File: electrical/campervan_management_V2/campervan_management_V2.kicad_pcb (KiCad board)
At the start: 4 copper layers, 169.5 x 96 mm, 172 parts, among them J1 Battery & Fuse, J10 Fans, J2 RS485, J3 Temp, J4 Output Flow Sensor, J5 Input Flow Sensor, J6 Power On/Off Switch, J7 Starter Battery, J8 Battery 2, J9 Relays, K1 G6KU-2, Q1 Q_PMOS_DGS, Q2 Q_PMOS_DGS, Q3 Q_PMOS_DGS, Q4 Q_PMOS_DGS, Q5 Q_PMOS_DGS, Q6 Q_PMOS_DGS, Q7 MMBT2222A, Q8 MMBT2222A, SW1 SW_Push, U1 MCP16311x-xMNY, U10 LM358DR2G, U11 LM358DR2G, U12 LTV-817S-TA1-C, U13 LTV-817S-TA1-C, U14 LTV-817S-TA1-C, U15 HCNR200-500E, U16 LTV-817S-TA1-C, U17 LM358DR2G, U18 LTV-817S-TA1-C, U19 LM358DR2G, U2 AMS1117-3.3, U20 LTV-817S-TA1-C, U21 LTV-817S-TA1-C, U22 HCNR200-500E, U23 LM358DR2G, U24 LTV-817S-TA1-C, U25 LTV-817S-TA1-C, U3 MCP16311x-xMNY, U4 AMS1117-3.3, U5 MAX487E, U6 LTV-817S-TA1-C, U7 LTV-817S-TA1-C, U8 LTV-817S-TA1-C, U9 HCNR200-500E

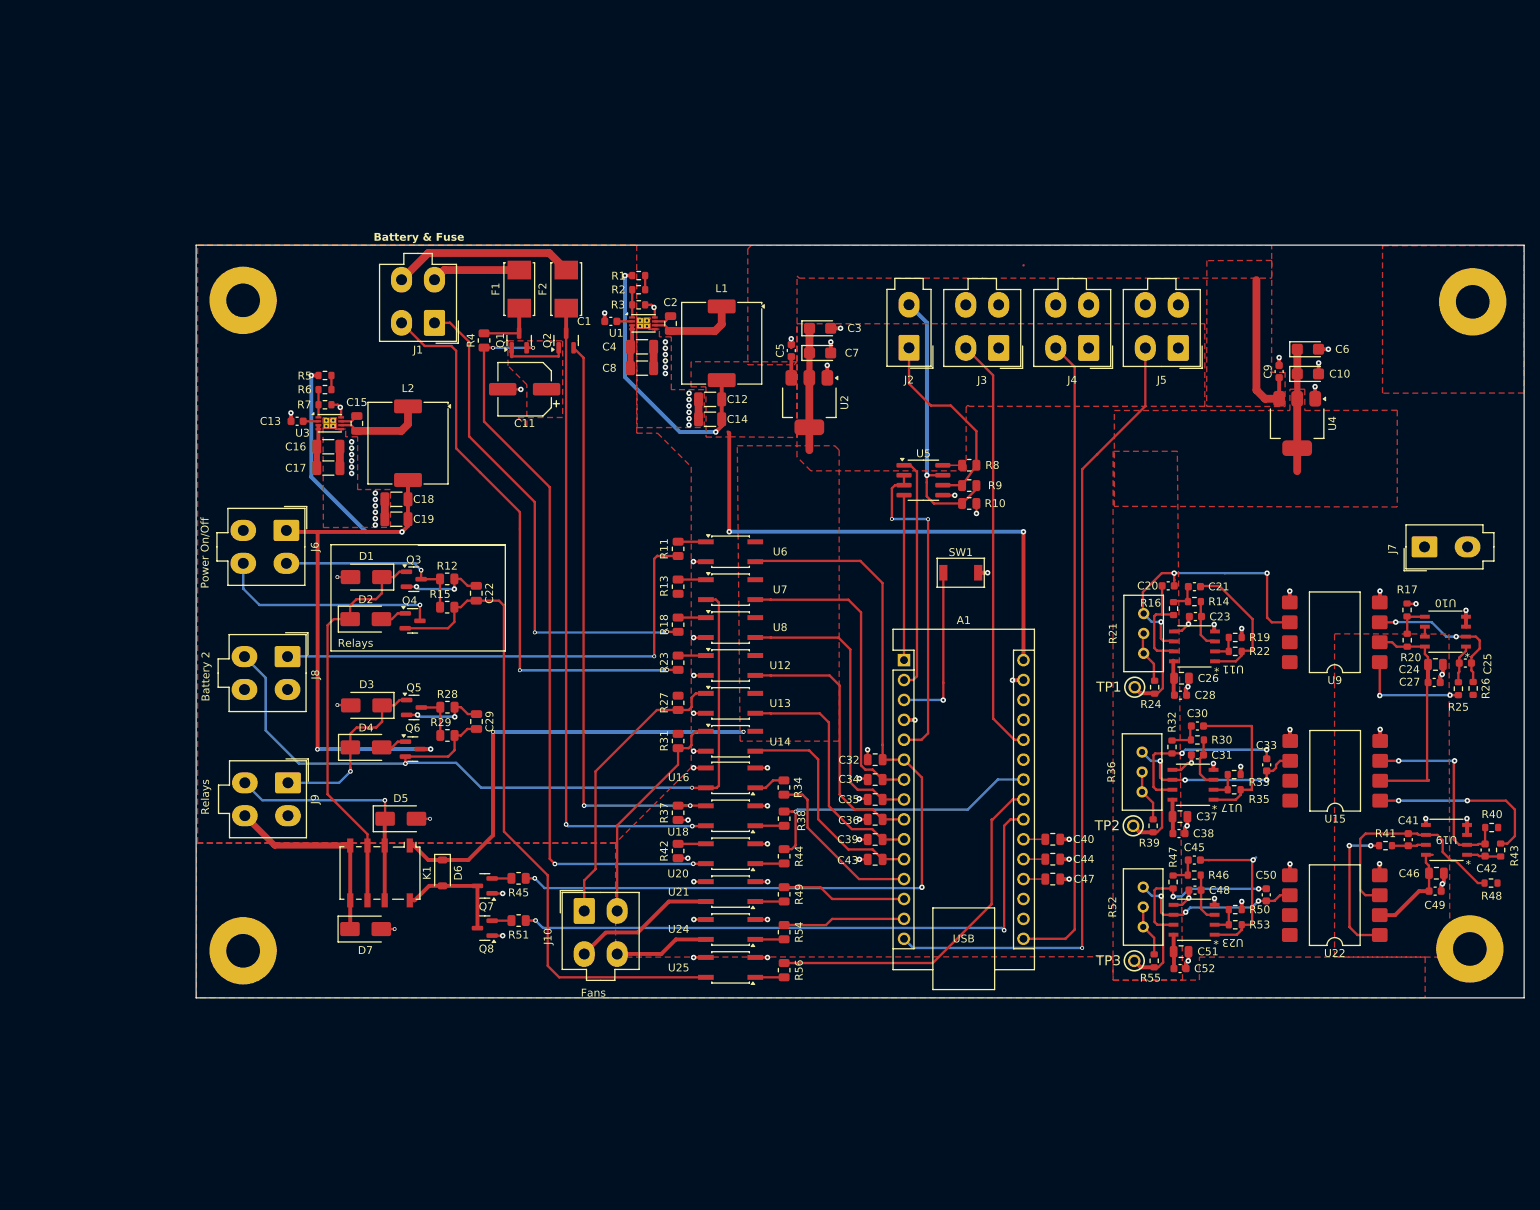
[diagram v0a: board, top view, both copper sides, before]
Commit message: Close to final design
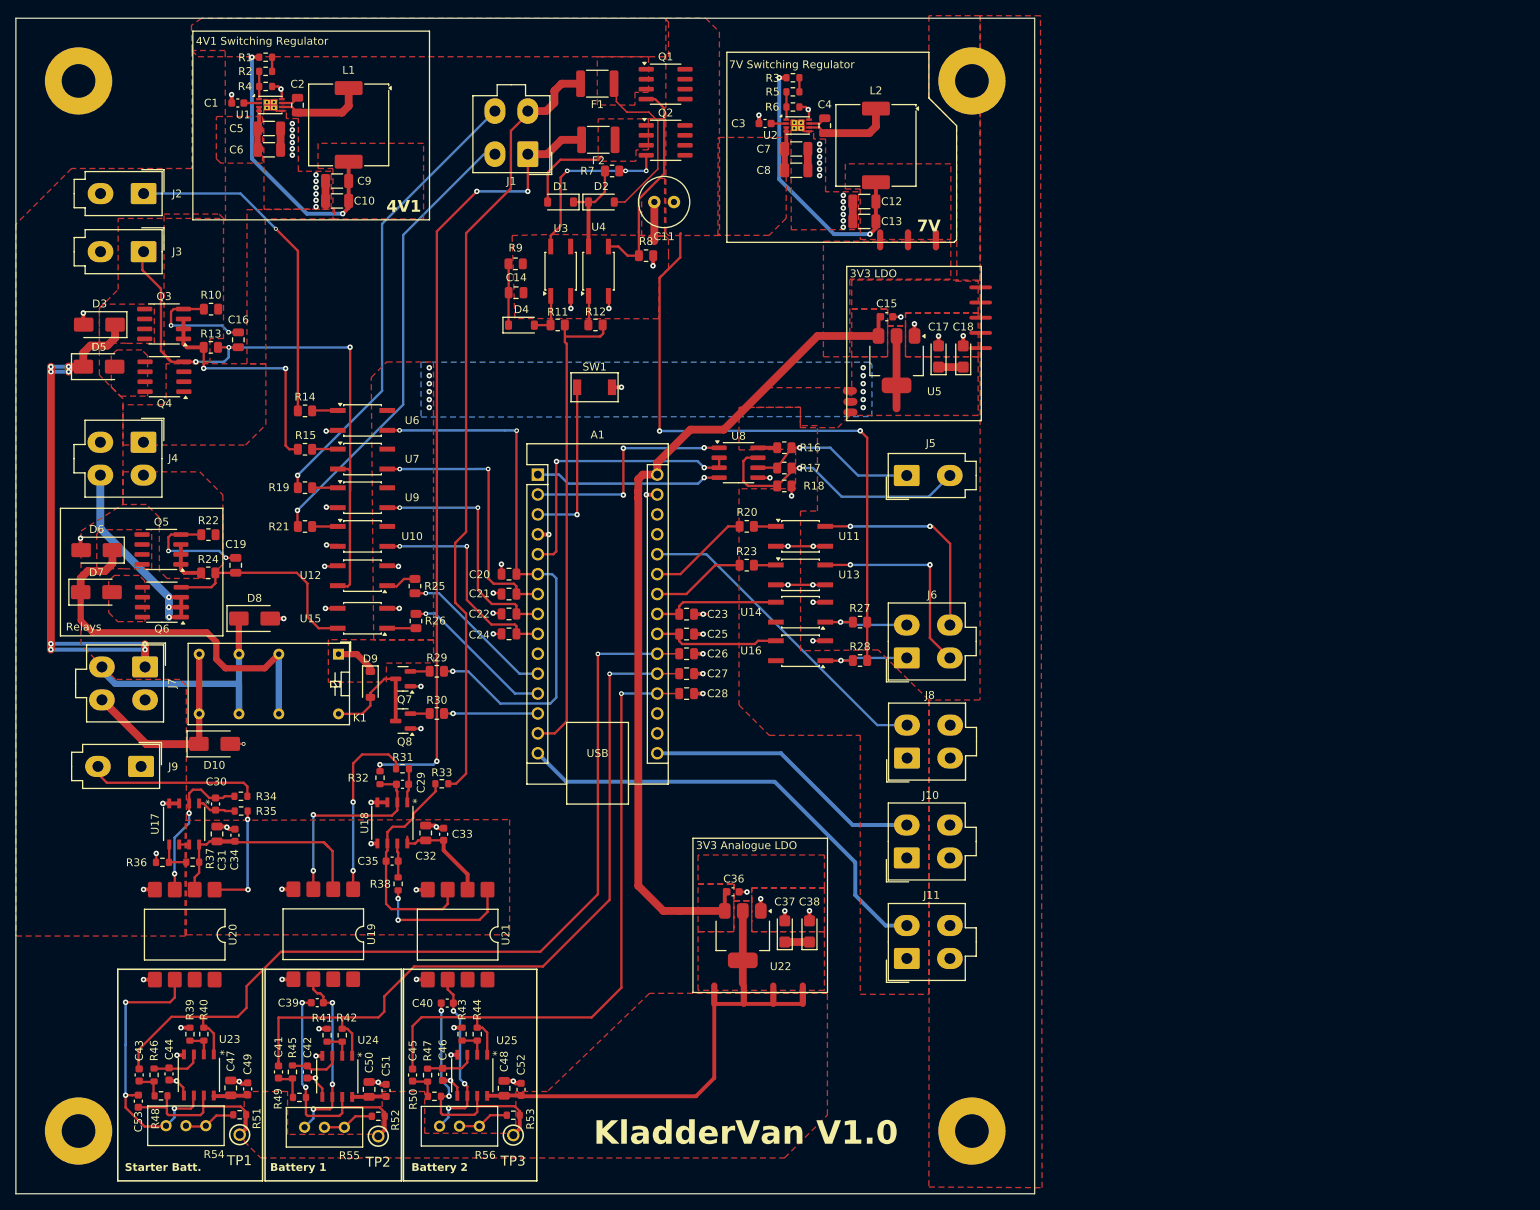
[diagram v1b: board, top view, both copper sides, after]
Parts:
- removed the J8 at (61.7, 106.5)
- removed the R42 at (111.5, 131.3)
- added C14: 220pF, Capacitor_SMD:C_0805_2012Metric, F.Cu at (90.8, 60.0)
- added D1: 1N418W, Diode_SMD:D_SOD-123, F.Cu at (96.5, 48.5)
- added D2: 1N418W, Diode_SMD:D_SOD-123, F.Cu at (101.7, 48.5)
- added D4: 1N418W, Diode_SMD:D_SOD-123, F.Cu at (91.5, 64.2)
- added J2: Battery 2, Connector_Molex:Molex_Mini-Fit_Jr_5566-02A_2x01_P4.20mm_Vertical, F.Cu at (43.3, 47.4)
- added J3: Solar Charge, Connector_Molex:Molex_Mini-Fit_Jr_5566-02A_2x01_P4.20mm_Vertical, F.Cu at (43.3, 54.8)
- added R9: 330, Resistor_SMD:R_0805_2012Metric, F.Cu at (90.8, 56.3)
- C11: footprint Capacitor_SMD:CP_Elec_6.3x5.9 -> Capacitor_THT:C_Radial_D6.3mm_H11.0mm_P2.50mm
- F1: renamed from F2; footprint Fuse:Fuseholder_Littelfuse_Nano2_157x -> Fuse:Fuse_1812_4532Metric
- F2: renamed from F1; footprint Fuse:Fuseholder_Littelfuse_Nano2_157x -> Fuse:Fuse_1812_4532Metric
- K1: value G6KU-2 -> G5V-2; footprint Relay_SMD:Relay_DPDT_Omron_G6K-2F-Y -> Relay_THT:Relay_DPDT_Omron_G5V-2
- Q1, Q2, Q3, Q4, Q5, Q6: value Q_PMOS_DGS -> FDS4685; footprint Package_TO_SOT_SMD:SOT-23 -> Package_SO:SOIC-8_3.9x4.9mm_P1.27mm
- R51: renamed from R24; value 22k -> 10k
- R52: renamed from R39; value 22k -> 10k
- R53: renamed from R55; value 22k -> 10k
- R7: renamed from R4; value 47k -> 1k
- R8: renamed from R37; value 47k -> 27k
- U22: renamed from U4; value AMS1117-3.3 -> AMS1117-3.3/TLV761
- U5: renamed from U2; value AMS1117-3.3 -> AMS1117-3.3/TLV761
- moved J9 166.2 mm to (43.0, 120.5), turned to -90 degrees
- moved U17 162.8 mm to (48.5, 127.8), turned to -90 degrees
- moved R36 162.0 mm to (45.7, 132.7), turned to 180 degrees
- moved C30 160.5 mm to (52.5, 125.3), turned to 90 degrees
- moved R34 157.8 mm to (55.7, 124.3), turned to 180 degrees
- moved R37 157.5 mm to (49.6, 132.7), turned to 180 degrees
- moved C31 157.0 mm to (52.7, 129.1), turned to 90 degrees
- moved R35 156.1 mm to (55.7, 126.2), turned to 0 degrees
- moved C34 154.3 mm to (55.0, 129.3), turned to 90 degrees
- moved U20 151.7 mm to (48.5, 141.9), turned to -90 degrees
- moved C43 148.4 mm to (42.7, 159.8), turned to 90 degrees
- moved C53 147.0 mm to (42.6, 163.2), turned to 90 degrees
- moved R46 145.9 mm to (44.6, 159.8), turned to 90 degrees
- moved C44 143.4 mm to (46.5, 159.7), turned to -90 degrees
- moved R48 143.4 mm to (45.5, 162.5), turned to 180 degrees
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- renumbered C13 to C1, C18 to C10, C14 to C13, C5 to C15, C29 to C16, C3 to C17, C7 to C18, C22 to C19, C15 to C2, C32 to C20, C34 to C21, C35 to C22, C43 to C23, C36 to C24, C39 to C25, C40 to C26, C44 to C27, C47 to C28, C42 to C29, C1 to C3, C25 to C30, C24 to C31, C46 to C32, C49 to C33, C27 to C34, C41 to C35, C9 to C36, C6 to C37, C10 to C38, C33 to C39, C2 to C4, C50 to C40, C30 to C41, C31 to C42, C21 to C43, C23 to C44, C48 to C46, C26 to C47, C51 to C48, C28 to C49, C16 to C5, C37 to C50, C38 to C51, C20 to C53, C17 to C6, C4 to C7, C19 to C9, D7 to D10, D4 to D5, D1 to D6, D2 to D7, D5 to D8, D6 to D9, H4 to H3, H3 to H4, J4 to J10, J5 to J11, J6 to J4, J2 to J5, J10 to J6, J9 to J7, J3 to J8, J7 to J9, L2 to L1, L1 to L2, R5 to R1, R28 to R10, R44 to R11, R38 to R12, R29 to R13, R11 to R14, R13 to R15, R8 to R16, R9 to R17, R10 to R18, R18 to R19, R6 to R2, R54 to R20, R23 to R21, R12 to R22, R49 to R23, R15 to R24, R34 to R25, R56 to R26, R31 to R27, R27 to R28, R45 to R29, R1 to R3, R51 to R30, R43 to R31, R40 to R32, R48 to R33, R26 to R34, R25 to R35, R17 to R36, R20 to R37, R41 to R38, R19 to R39, R7 to R4, R22 to R40, R33 to R41, R35 to R42, R50 to R43, R53 to R44, R30 to R45, R14 to R46, R46 to R47, R16 to R48, R32 to R49, R2 to R5, R47 to R50, R21 to R54, R36 to R55, R52 to R56, R3 to R6, U3 to U1, U12 to U10, U24 to U11, U16 to U12, U21 to U13, U25 to U15, U13 to U16, U10 to U17, U19 to U18, U15 to U19, U1 to U2, U9 to U20, U22 to U21, U11 to U23, U17 to U24, U23 to U25, U20 to U3, U18 to U4, U5 to U8, U8 to U9
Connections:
- A1 pad 10: /Battery Box Fan2 Sensor -> unconnected-(A1-D7-Pad10)
- A1 pad 11: /Battery Box Fan1 Sensor -> /Solar Charge Management/Solar Charge Battery 2 On
- A1 pad 12: /Solar Charge Management/Solar Charge Battery 2 On -> /Batteries On
- A1 pad 13: /Battery Box Fan1 Control -> /Battery 2 On/Off
- A1 pad 14: /Battery Box Fan2 Control -> /Power Supply Control
- A1 pad 19: /Battery Voltage Measurement/Starter Battery Voltage -> /Battery Voltage Measurement/Battery 2 Voltage
- A1 pad 21: /Battery Voltage Measurement/Battery 2 Voltage -> /Battery Voltage Measurement/Starter Battery Voltage
- A1 pad 22: /Battery 2 On/Off -> /Battery Box Fan2 Sensor
- A1 pad 23: /Batteries On -> /Battery Box Fan1 Sensor
- A1 pad 24: /Power Supply Control -> /Battery Box Fan1 Control
- A1 pad 25: unconnected-(A1-A6-Pad25) -> /Battery Box Fan2 Control
- C16 pad 1: Net-(Q7-G) -> Net-(Q3-G)
- C19 pad 1: Net-(Q2-G) -> Net-(Q5-G)
- C19 pad 2: Net-(Q1-G) -> Net-(Q6-G)
- C26 pad 1: /Battery Voltage Measurement/Battery 2 Voltage -> /Battery Voltage Measurement/Starter Battery Voltage
- C28 pad 1: /Battery Voltage Measurement/Starter Battery Voltage -> /Battery Voltage Measurement/Battery 2 Voltage
- D5 pad 2: Net-(D2-A) -> /Solar Charge Management/test
- D6 pad 1: Net-(D5-K) -> Net-(D6-K)
- D7 pad 1: Net-(D5-K) -> Net-(D6-K)
- D7 pad 2: Net-(D5-A) -> Net-(D7-A)
- D9 pad 2: Net-(D6-A) -> Net-(D9-A)
- F1 pad 1: Net-(Q8-S) -> Net-(D2-A)
- F1 pad 2: /Battery Voltage Measurement/Battery 1 Vin -> /Battery Voltage Measurement/Battery 2 Vin
- F2 pad 1: Net-(Q9-S) -> Net-(D1-A)
- F2 pad 2: /Battery Voltage Measurement/Battery 2 Vin -> /Battery Voltage Measurement/Battery 1 Vin
- J1 pad 1: /Battery Fuse Sensors/Battery 1 Fuse Sensor -> /Battery Voltage Measurement/Battery 1 Vin
- J1 pad 4: /Battery Voltage Measurement/Battery 1 Vin -> /Battery Fuse Sensors/Battery 1 Fuse Sensor
- K1 pad 4: /Battery Management/Battery 1 Relay -> Net-(D6-K)
- K1 pad 6: Net-(D5-K) -> /Battery Management/Battery 2 Relay
- K1 pad 8: Net-(D6-A) -> /Battery Management/Battery 1 Relay
- Q1 pad 1: VIN -> Net-(D2-A)
- Q1 pad 2: Net-(Q9-G) -> Net-(D2-A)
- Q1 pad 3: Net-(Q9-S) -> Net-(D2-A)
- Q2 pad 1: VIN -> Net-(D1-A)
- Q2 pad 2: Net-(Q8-G) -> Net-(D1-A)
- Q2 pad 3: Net-(Q8-S) -> Net-(D1-A)
- Q3 pad 1: Net-(D5-K) -> VIN
- Q3 pad 2: Net-(Q2-G) -> VIN
- Q3 pad 3: /Battery Management/Power On Switch - 4V1 -> VIN
- Q4 pad 1: Net-(D5-A) -> VCC_4V1
- Q4 pad 2: Net-(Q1-G) -> VCC_4V1
- Q4 pad 3: /Battery Management/Power On Switch - Vin -> VCC_4V1
- Q5 pad 1: /Solar Charge Battery 2 Relay -> /Battery Management/Power On Switch - 4V1
- Q5 pad 2: Net-(Q7-G) -> /Battery Management/Power On Switch - 4V1
- Q5 pad 3: VIN -> /Battery Management/Power On Switch - 4V1
- Q6 pad 1: Net-(D2-A) -> /Battery Management/Power On Switch - Vin
- Q6 pad 2: /Solar Charge Management/Solar Charge Battery 2 Switch -> /Battery Management/Power On Switch - Vin
- Q6 pad 3: VCC_4V1 -> /Battery Management/Power On Switch - Vin
- Q7 pad 3: Net-(D6-A) -> Net-(D9-A)
- Q8 pad 3: Net-(D6-A) -> Net-(D9-A)
- R10 pad 2: Net-(Q7-G) -> Net-(Q3-G)
- R22 pad 2: Net-(Q2-G) -> Net-(Q5-G)
- R24 pad 2: Net-(Q1-G) -> Net-(Q6-G)
- R7 pad 1: Net-(Q9-S) -> /Power Supply/Vps
- R7 pad 2: Net-(Q9-G) -> Net-(Q2-G)
- R8 pad 1: Net-(Q8-G) -> Net-(Q1-G)
- U15 pad 4: Net-(Q1-G) -> Net-(Q6-G)
- U3 pad 3: Net-(R57-Pad1) -> GND
- U3 pad 4: Net-(Q9-G) -> Net-(Q2-G)
- U4 pad 3: Net-(Q8-G) -> Net-(Q1-G)
- U4 pad 4: Net-(Q8-S) -> /Power Supply/Vps
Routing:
- net VIN: track 69.6 -> 166.9 mm, vias 0 -> 4
- net /Battery Voltage Measurement/Starter Battery Voltage: track 21.1 -> 117.7 mm, vias 0 -> 1
- net Net-(Q9-G): track 96.1 -> 0.00 mm, vias 4 -> 0
- net /Battery Voltage Measurement/Battery 2 Vin: track 11.3 -> 100.2 mm
- net Net-(Q8-S): track 83.8 -> 0.00 mm, vias 2 -> 0
- net /Battery Voltage Measurement/Battery 1 Vin: track 23.3 -> 101.7 mm, vias 0 -> 4
- net /Battery Voltage Measurement/Battery 1 Voltage: track 23.0 -> 99.3 mm, vias 0 -> 1
- net Net-(Q8-G): track 76.1 -> 0.00 mm, vias 2 -> 0
- net /Battery 2 On/Off: track 77.7 -> 12.0 mm, vias 2 -> 1
- net /Battery Voltage Measurement/Battery 2 Voltage: track 24.2 -> 84.8 mm
- net VCC_4V1: track 93.7 -> 35.3 mm, vias 4 -> 2
- net Net-(Q1-G): track 84.5 -> 27.5 mm
- net /Solar Charge Battery 2 Relay: track 23.6 -> 78.4 mm, vias 1 -> 8
- net VCC_3V3: track 75.9 -> 22.5 mm, vias 2 -> 12
- net Net-(D5-K): track 52.3 -> 0.00 mm
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- added copper zone on F.Cu, net /Battery Management/Power On Switch - 4V1
- added copper zone on F.Cu, net /Solar Charge Battery 2 Relay
- added copper zone on F.Cu, net /Solar Charge Management/test
- added copper zone on F.Cu, net Net-(D1-A)
- added copper zone on F.Cu, net Net-(D2-A)
- added copper zone on F.Cu, net Net-(D6-K)
- added copper zone on F.Cu, net Net-(D7-A)
- added copper zone on B.Cu, net VCC_3V3
- added copper zone on F.Cu, net VCC_4V1
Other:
- board size 169.5 x 96 mm -> 130 x 150 mm
- board text added: "3V3 Analogue LDO"
- board text added: "4V1"
- board text added: "7V"
- board text added: "Battery 1"
- board text added: "KladderVan V1.0"
- board text added: "Starter Batt."
- board text removed: "Battery & Fuse"
- board text removed: "Fans"
- board text removed: "Power On/Off"
